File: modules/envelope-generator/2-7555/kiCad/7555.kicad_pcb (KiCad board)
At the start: 2 copper layers, 81 x 111 mm, 89 parts, among them J1 JUMPER_BUS_GATE, J2 PWR, Q1 BC547, Q2 BC547, Q3 BC547, SW1 SW_SPDT, U1 TL074, U2 ICM7555xP

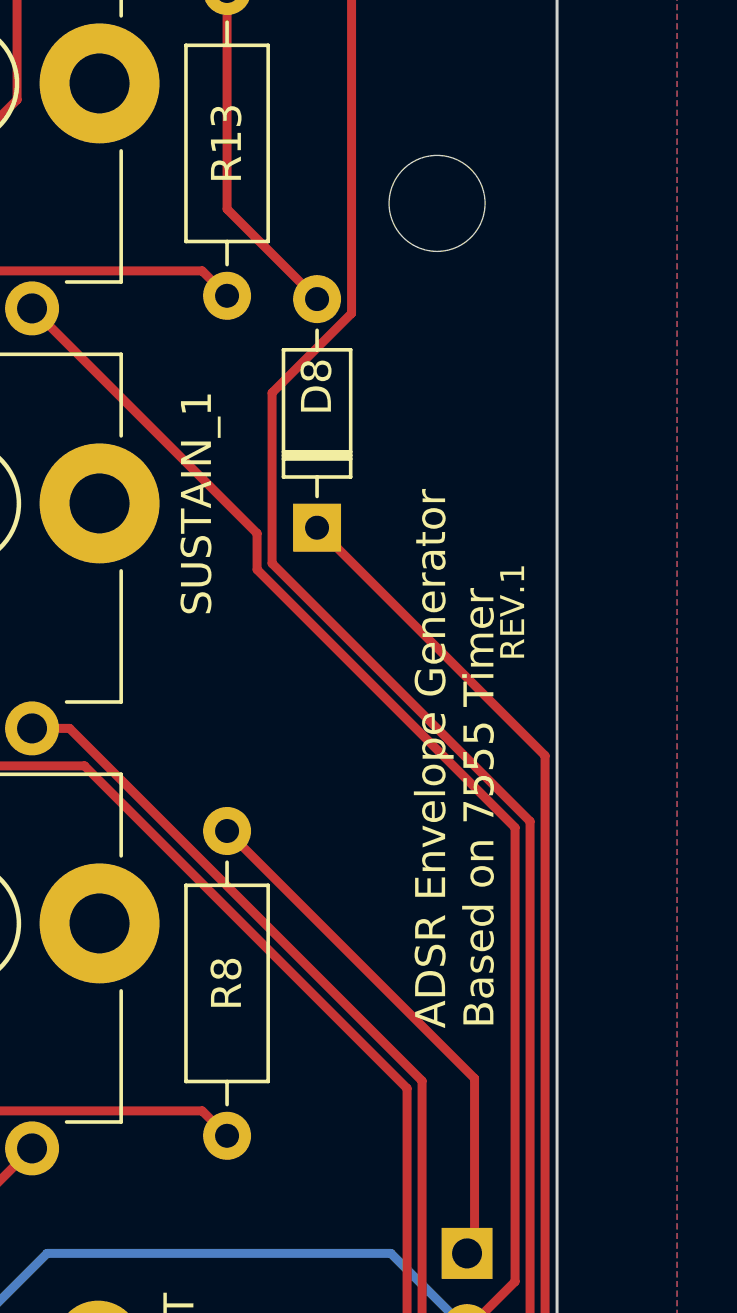
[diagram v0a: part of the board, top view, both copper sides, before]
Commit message: final versions of PCB for modules
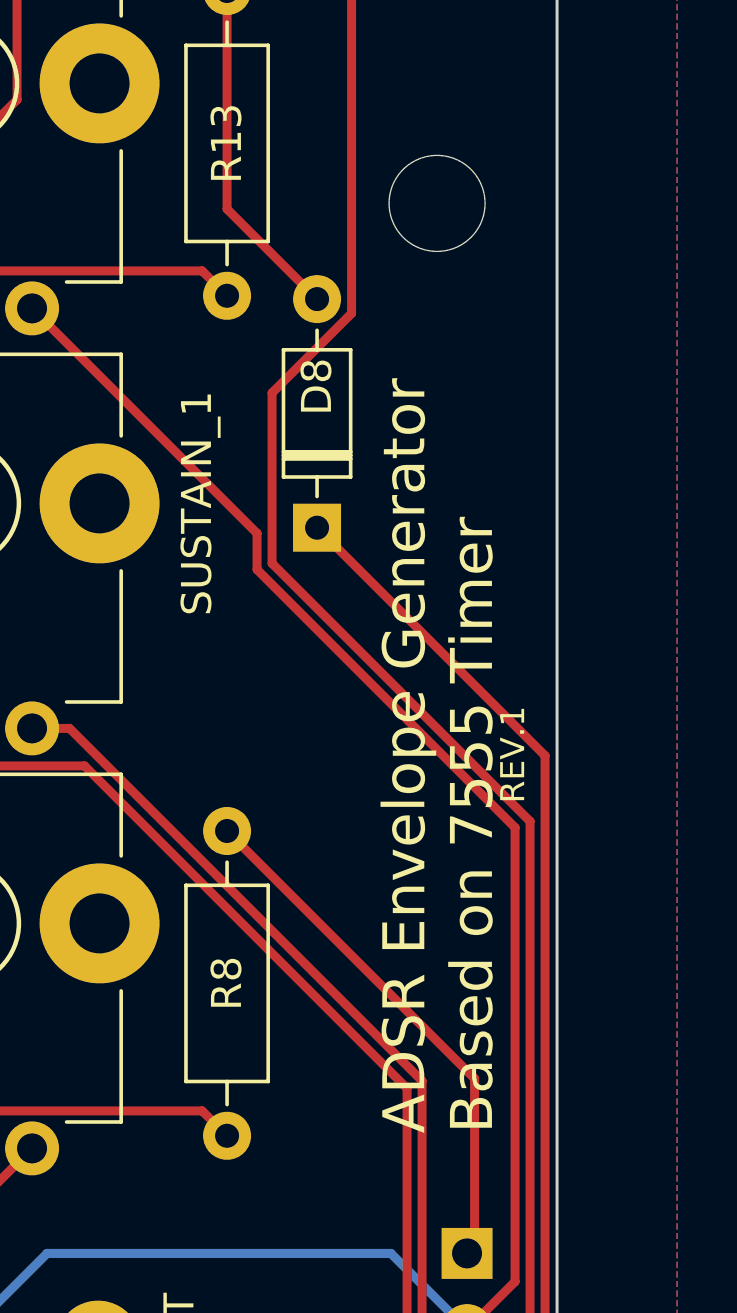
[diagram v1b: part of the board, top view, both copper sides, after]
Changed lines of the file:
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@@
 		(grid_origin 50 50)
 		(pcbplotparams
-			(layerselection 0x00010fc_ffffffff)
+			(layerselection 0x00410fc_ffffffff)
 			(plot_on_all_layers_selection 0x0000000_00000000)
 			(disableapertmacros no)
-			(usegerberextensions no)
-			(usegerberattributes yes)
-			(usegerberadvancedattributes yes)
-			(creategerberjobfile yes)
+			(usegerberextensions yes)
+			(usegerberattributes no)
+			(usegerberadvancedattributes no)
+			(creategerberjobfile no)
 			(dashed_line_dash_ratio 12.000000)
 			(dashed_line_gap_ratio 3.000000)
@@
 			(psa4output no)
 			(plotreference yes)
-			(plotvalue yes)
+			(plotvalue no)
 			(plotfptext yes)
 			(plotinvisibletext no)
 			(sketchpadsonfab no)
-			(subtractmaskfromsilk no)
+			(subtractmaskfromsilk yes)
 			(outputformat 1)
 			(mirror no)
-			(drillshape 1)
+			(drillshape 0)
 			(scaleselection 1)
-			(outputdirectory "")
+			(outputdirectory "../gerbers/")
 		)
 	)
@@
 	)
 	(gr_text "REV.1"
-		(at 130 90.25 90)
+		(at 130 95 90)
 		(layer "F.SilkS")
 		(effects
@@
 	)
 	(gr_text "ADSR Envelope Generator\nBased on 7555 Timer"
-		(at 129 102.5 90)
+		(at 129 106 90)
 		(layer "F.SilkS")
 		(effects
 			(font
-				(size 1 1)
+				(size 1.4 1.4)
 				(thickness 0.15)
 			)
